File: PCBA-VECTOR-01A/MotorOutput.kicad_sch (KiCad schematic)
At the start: 3 parts, among them J10 Conn_02x06_Odd_Even, J11 Conn_02x06_Odd_Even, J9 Conn_02x06_Odd_Even

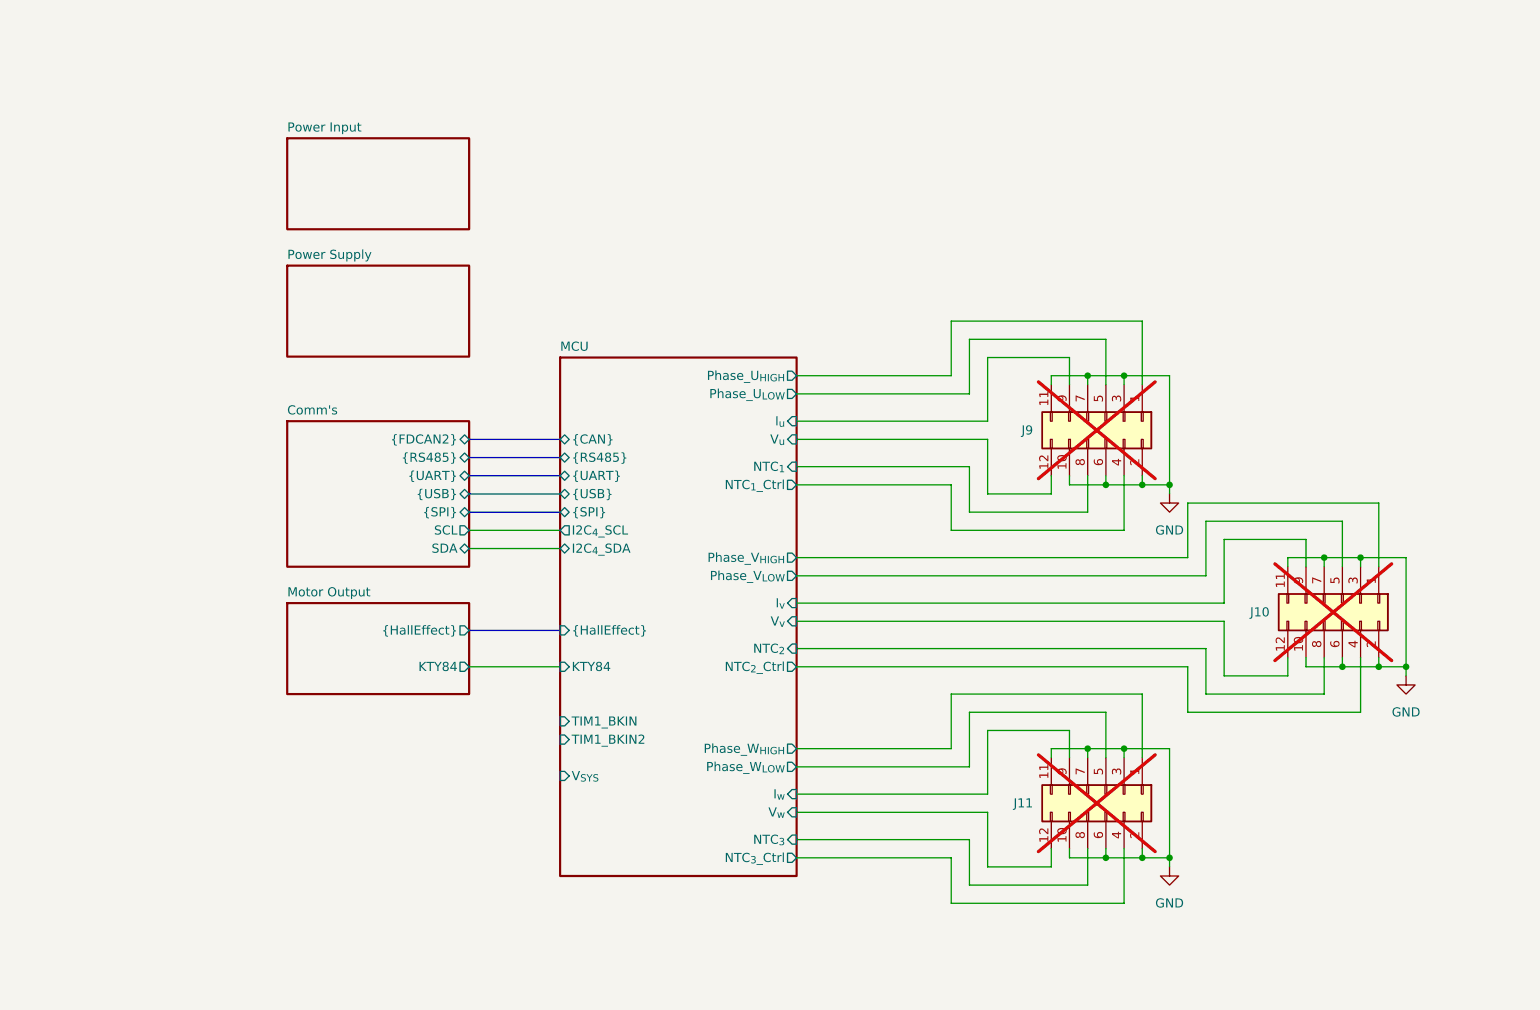
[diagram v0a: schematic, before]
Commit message: Changes were made
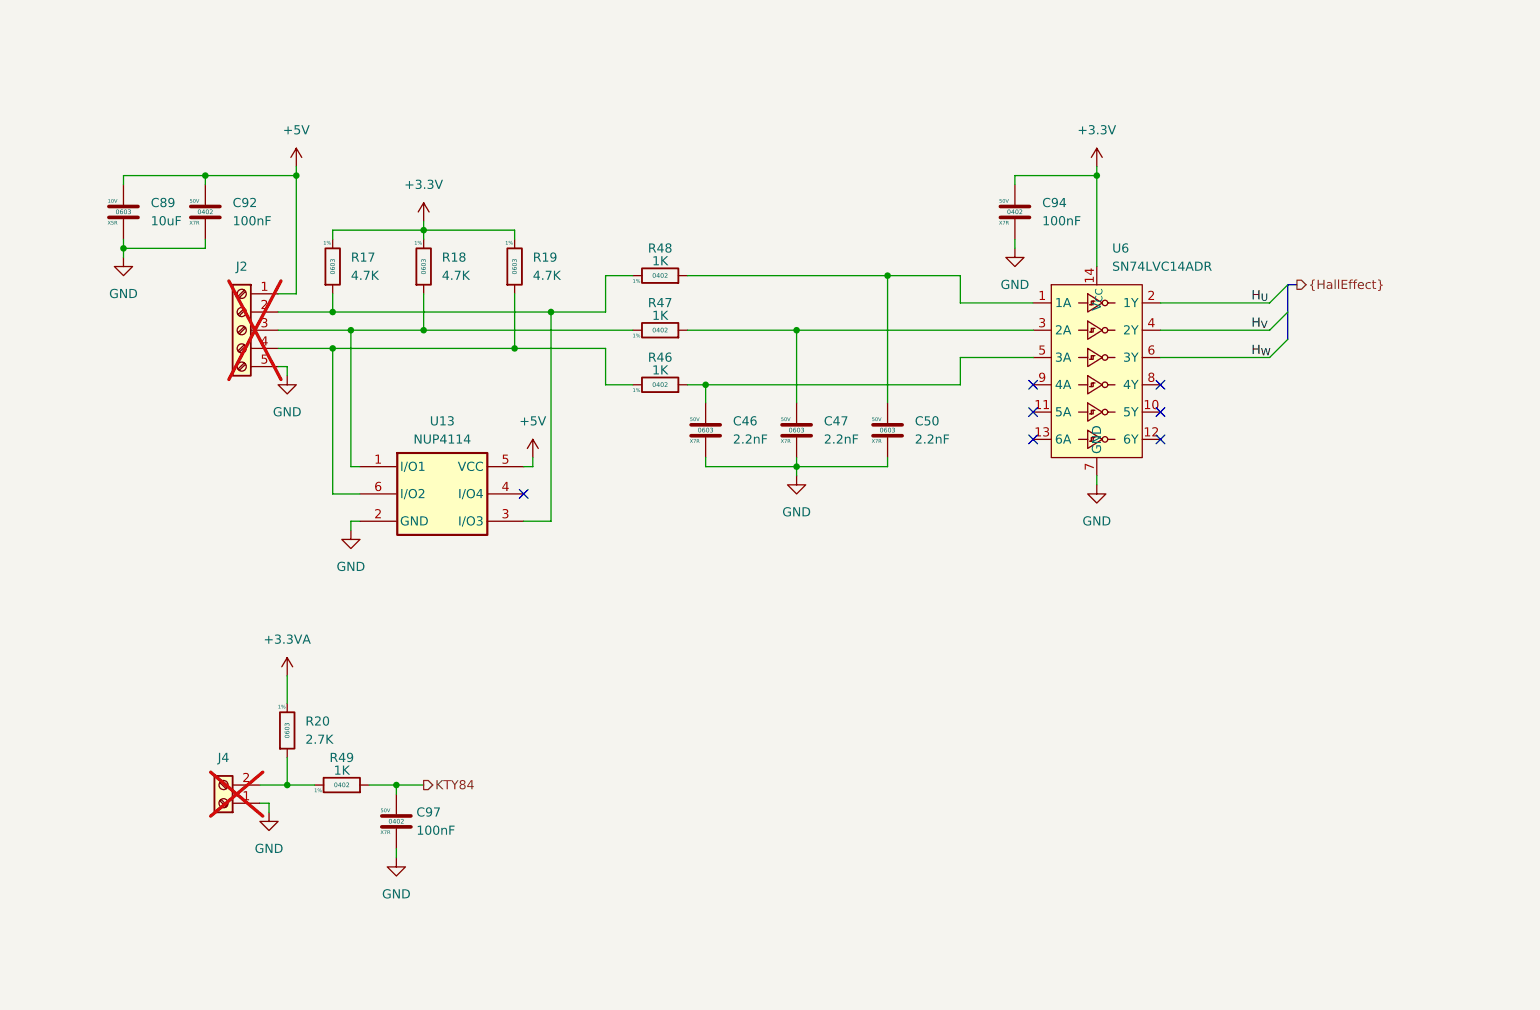
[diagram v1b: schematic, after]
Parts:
- removed J10, J11, J9: Conn_02x06_Odd_Even, Connector_PinHeader_2.54mm:PinHeader_2x06_P2.54mm_Vertical, symbol Connector_Generic:Conn_02x06_Odd_Even
- added C46, C47, C50: 2.2nF, Capacitor_SMD:C_0603_1608Metric, symbol Device:C
- added C89: 10uF, Capacitor_SMD:C_0603_1608Metric, symbol Device:C
- added C92, C94, C97: 100nF, Capacitor_SMD:C_0402_1005Metric, symbol Device:C
- added J2: Screw_Terminal_01x05, Bvrny's_library:TerminalBlock_5.08_01x05_JLAB, symbol Connector:Screw_Terminal_01x05
- added J4: Screw_Terminal_01x02, Bvrny's_library:TerminalBlock_5.08_01x02_JLAB, symbol Connector:Screw_Terminal_01x02
- added R17, R18, R19: 4.7K, Resistor_SMD:R_0603_1608Metric, symbol Device:R
- added R20: 2.7K, Resistor_SMD:R_0603_1608Metric, symbol Device:R
- added R46, R47, R48, R49: 1K, Resistor_SMD:R_0402_1005Metric, symbol Device:R
- added U13: NUP4114, Package_SO:TSOP-6_1.65x3.05mm_P0.95mm, symbol Bvrny's_library:NUP4114
- added U6: SN74LVC14ADR, Package_SO:SOIC-14_3.9x8.7mm_P1.27mm, symbol Bvrny's_library:SN74LVC14ADR
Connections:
- net GND: now also C46.2, C47.2, C50.2, C89.2, C92.2, C94.2, C97.2, J2.5 (Pin_5), J4.1 (Pin_1), U13.2 (GND), U6.7 (GND)
- new net: C50.1, R48.2, U6.1 (1A)
- new net: C47.1, R47.2, U6.3 (2A)
- new net: C46.1, R46.2, U6.5 (3A)
- new net: J2.4 (Pin_4), R19.2, R46.1, U13.6 (I/O2)
- new net: J4.2 (Pin_2), R20.2, R49.1
- new net: J2.2 (Pin_2), R17.2, R48.1, U13.3 (I/O3)
- new net: J2.3 (Pin_3), R18.2, R47.1, U13.1 (I/O1)
- new net +3.3V: C94.1, R17.1, R18.1, R19.1, U6.14 (V_{CC})
- new net +3.3VA: R20.1
- new net +5V: C89.1, C92.1, J2.1 (Pin_1), U13.5 (VCC)
- new net H_{U}: U6.2 (1Y)
- new net H_{V}: U6.4 (2Y)
- new net H_{W}: U6.6 (3Y)
- new net KTY84: C97.1, R49.2
- no-connect marks 0 -> 7
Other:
- removed sheet Comm's
- removed sheet MCU
- removed sheet Motor Output
- removed sheet Power Input
- removed sheet Power Supply

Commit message: Finished schematic?
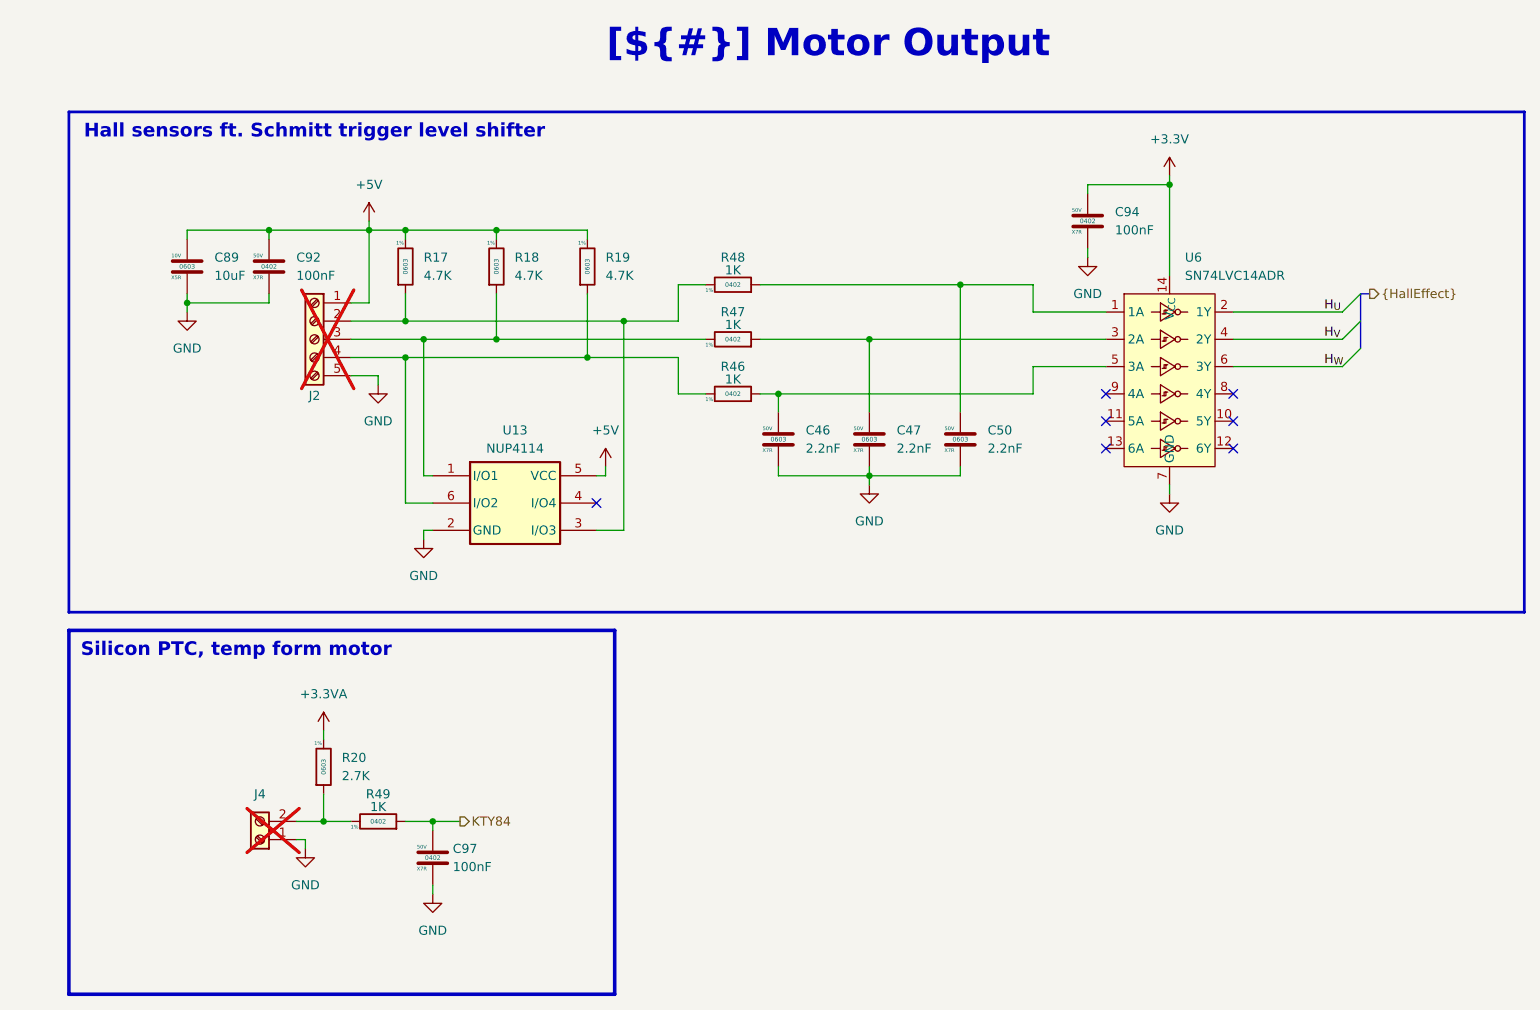
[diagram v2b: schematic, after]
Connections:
- net +3.3V: no longer R17.1, R18.1, R19.1
- net +5V: now also R17.1, R18.1, R19.1
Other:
- note added: "Hall sensors ft. Schmitt trigger level shifter"
- note added: "Silicon PTC, temp form motor"
- moved on the sheet: C46, C47, C50, C89, C92, C94, C97, J2, J4, R17, R18, R19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
